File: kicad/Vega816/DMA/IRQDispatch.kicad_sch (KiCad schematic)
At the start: 15 parts, among them J14 DMA 0 IRQ, J15 DMA 1 IRQ, U1 74HC00, U12 74HC00, U14 74HC00, U24 74HC00, U25 74LS348, U26 74HC00, U27 74LS348, U28 74HC00, U29 74HC00, U8 74HC00, U9 74HC00

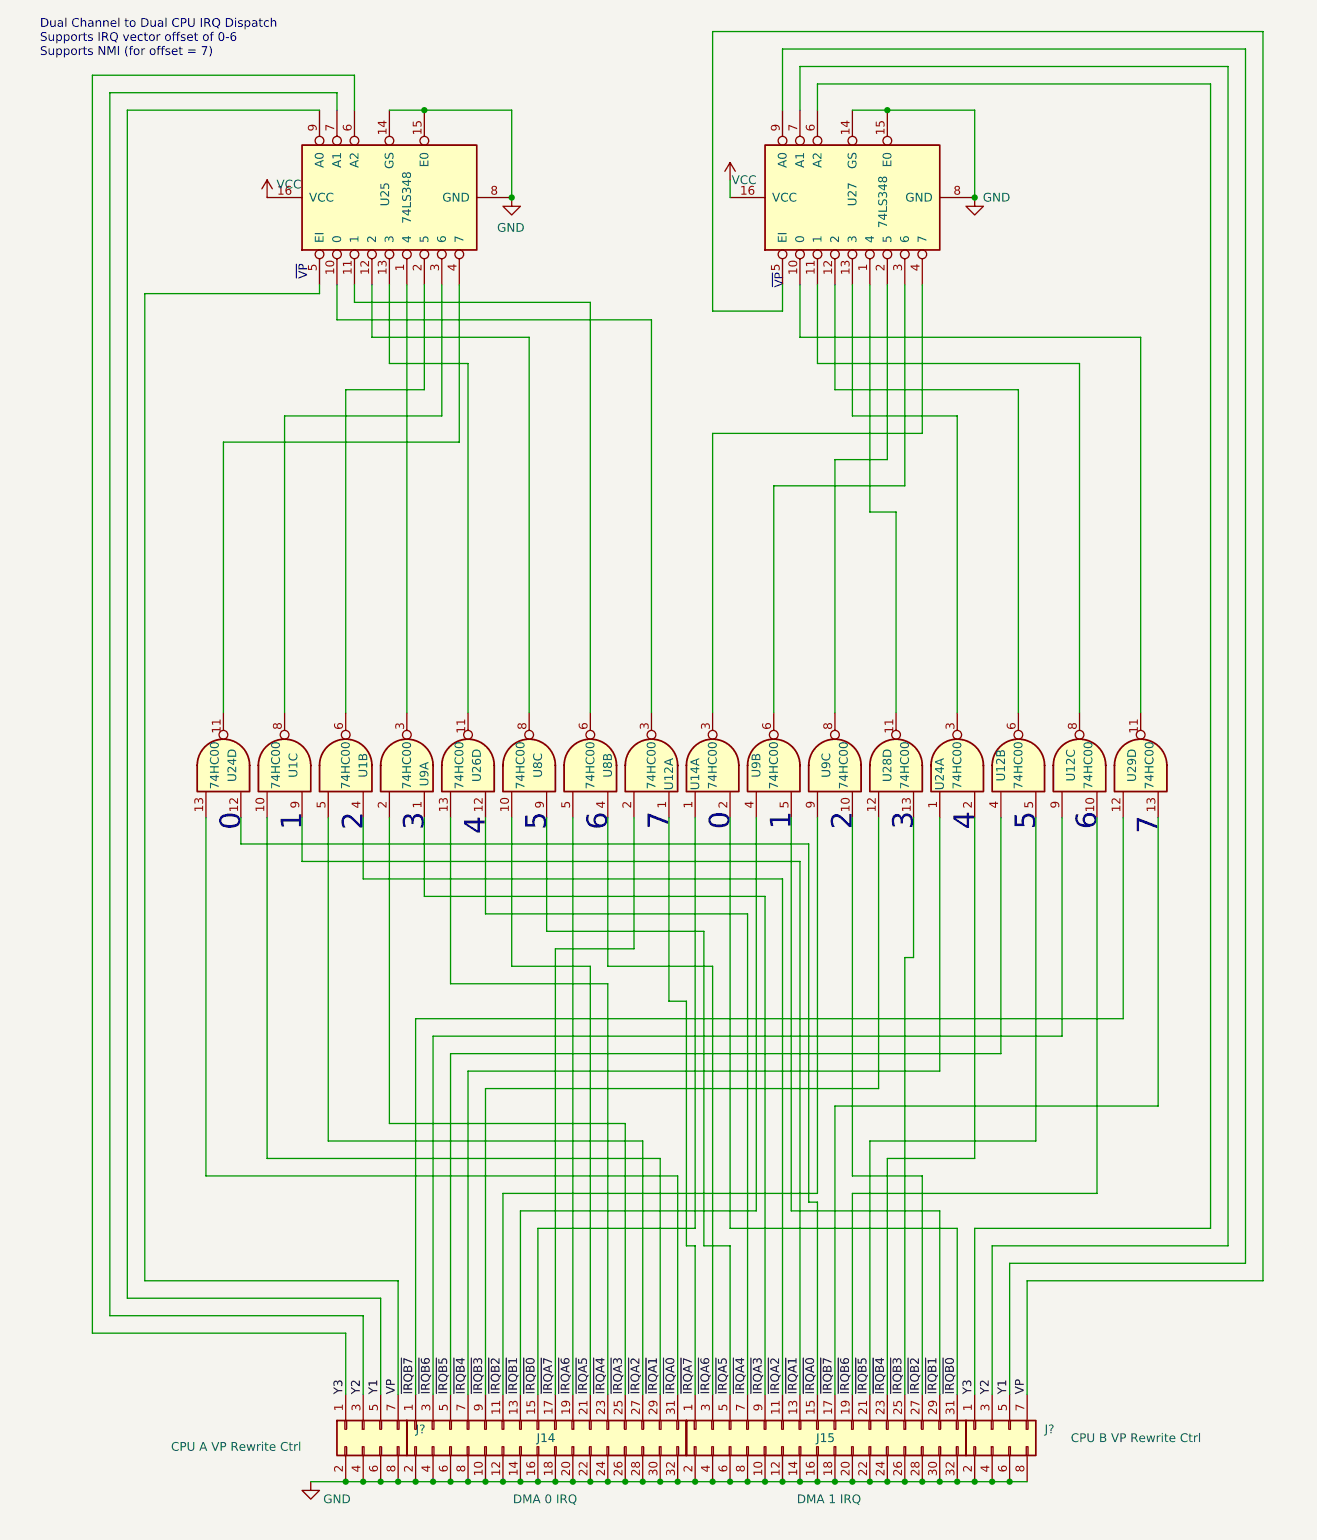
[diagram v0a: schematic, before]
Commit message: irq
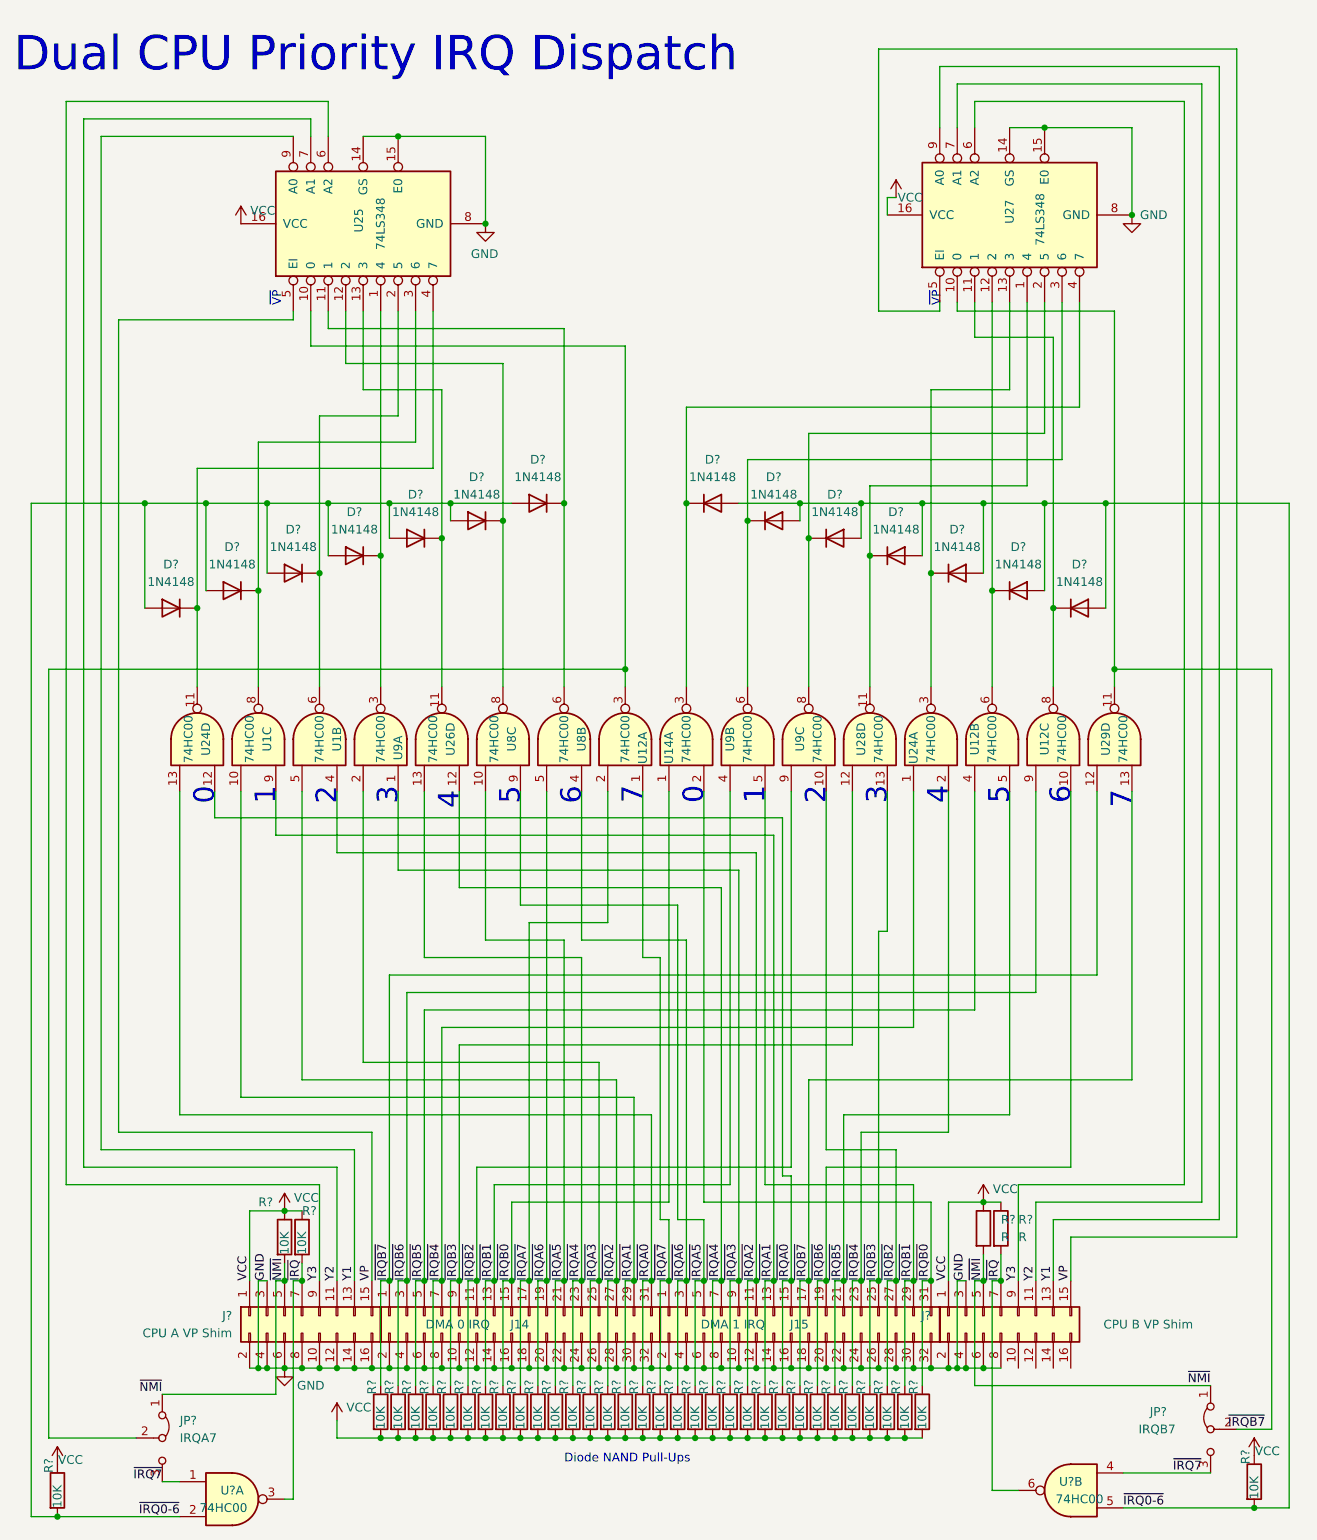
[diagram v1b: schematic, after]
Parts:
- removed J?: CPU A VP Rewrite Ctrl, symbol Connector_Generic:Conn_02x04_Odd_Even
- removed J?: CPU B VP Rewrite Ctrl, symbol Connector_Generic:Conn_02x04_Odd_Even
- added D? (x14): 1N4148, Diode_THT:D_DO-35_SOD27_P7.62mm_Horizontal, symbol Diode:1N4148
- added J?: CPU A VP Shim, symbol Connector_Generic:Conn_02x08_Odd_Even
- added J?: CPU B VP Shim, symbol Connector_Generic:Conn_02x08_Odd_Even
- added JP?: IRQA7, symbol Jumper:Jumper_3_Bridged12
- added JP?: IRQB7, symbol Jumper:Jumper_3_Bridged12
- added R? (x36): 10K, symbol Device:R
- added R? (x2): R, symbol Device:R
- added U? (x2): 74HC00, symbol 74xx:74HC00
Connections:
- net GND: now also J?.10 (Pin_10), J?.12 (Pin_12), J?.14 (Pin_14), J?.16 (Pin_16), J?.2 (Pin_2), J?.2 (Pin_2), J?.3 (Pin_3), J?.3 (Pin_3), J?.4 (Pin_4), J?.4 (Pin_4), J?.6 (Pin_6), J?.6 (Pin_6), J?.8 (Pin_8), J?.8 (Pin_8)
- net VCC: now also J?.1 (Pin_1), J?.1 (Pin_1), R?.1, R?.1, R?.1, R?.1, R?.1, R?.1, R?.2, R?.2, R?.2, R?.2, R?.2, R?.2, R?.2, R?.2, R?.2, R?.2, R?.2, R?.2, R?.2, R?.2, R?.2, R?.2, R?.2, R?.2, R?.2, R?.2, R?.2, R?.2, R?.2, R?.2, R?.2, R?.2, R?.2, R?.2, R?.2, R?.2, R?.2, R?.2
- net VP: now also J?.15 (Pin_15), J?.15 (Pin_15)
- net Y1: now also J?.13 (Pin_13), J?.13 (Pin_13)
- net Y2: now also J?.11 (Pin_11), J?.11 (Pin_11)
- net Y3: now also J?.9 (Pin_9), J?.9 (Pin_9)
- net ~{IRQA0}: now also R?.1, R?.1
- net ~{IRQA1}: now also R?.1, R?.1
- net ~{IRQA2}: now also R?.1, R?.1
- net ~{IRQA3}: now also R?.1, R?.1
- net ~{IRQA4}: now also R?.1, R?.1
- net ~{IRQA5}: now also R?.1, R?.1
- net ~{IRQA6}: now also R?.1, R?.1
- net ~{IRQA7}: now also R?.1, R?.1
- net ~{IRQB0}: now also R?.1, R?.1
- net ~{IRQB1}: now also R?.1, R?.1
- net ~{IRQB2}: now also R?.1, R?.1
- net ~{IRQB3}: now also R?.1, R?.1
- net ~{IRQB4}: now also R?.1, R?.1
- net ~{IRQB5}: now also R?.1, R?.1
- net ~{IRQB6}: now also R?.1, R?.1
- net ~{IRQB7}: now also R?.1, R?.1
- net at U27.1 (4), U28.11: now also D?.1 (K)
- net at U27.10 (0), U29.11: now also JP?.2 (C)
- net at U12.8, U27.11 (1): now also D?.1 (K)
- net at U12.6, U27.12 (2): now also D?.1 (K)
- net at U24.3, U27.13 (3): now also D?.1 (K)
- net at U27.2 (5), U9.8: now also D?.1 (K)
- net at U27.3 (6), U9.6: now also D?.1 (K)
- net at U14.3, U27.4 (7): now also D?.1 (K)
- net at U25.13 (3), U26.11: now also D?.1 (K)
- net at U25.1 (4), U9.3: now also D?.1 (K)
- net at U24.11, U25.4 (7): now also D?.1 (K)
- net at U1.8, U25.3 (6): now also D?.1 (K)
- net at U25.11 (1), U8.6: now also D?.1 (K)
- net at U25.12 (2), U8.8: now also D?.1 (K)
- net at U1.6, U25.2 (5): now also D?.1 (K)
- net at U12.3, U25.10 (0): now also JP?.2 (C)
- new net ~{IRQ0-6}: D?.2 (A), D?.2 (A), D?.2 (A), D?.2 (A), D?.2 (A), D?.2 (A), D?.2 (A), D?.2 (A), D?.2 (A), D?.2 (A), D?.2 (A), D?.2 (A), D?.2 (A), D?.2 (A), R?.2, R?.2, U?.2, U?.5
- new net ~{IRQ7}: JP?.3 (B), JP?.3 (B), U?.1, U?.4
- new net ~{IRQ}: J?.7 (Pin_7), J?.7 (Pin_7), R?.2, R?.2, U?.3, U?.6
- new net ~{NMI}: J?.5 (Pin_5), J?.5 (Pin_5), JP?.1 (A), JP?.1 (A), R?.2, R?.2
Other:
- note added: "Diode NAND Pull-Ups"
- note added: "Dual CPU Priority IRQ Dispatch"
- note removed: "Dual Channel to Dual CPU IRQ Dispatch Supports IRQ vector offset of 0-6 Supports NMI (for offset = 7)"
- moved on the sheet: J14, J15, U12A, U12B, U12C, U14A, U1B, U1C, U24A, U24D, U25, U26D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
